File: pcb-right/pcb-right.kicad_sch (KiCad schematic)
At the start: 39 parts, among them J3 BAT, U2 xiao-ble

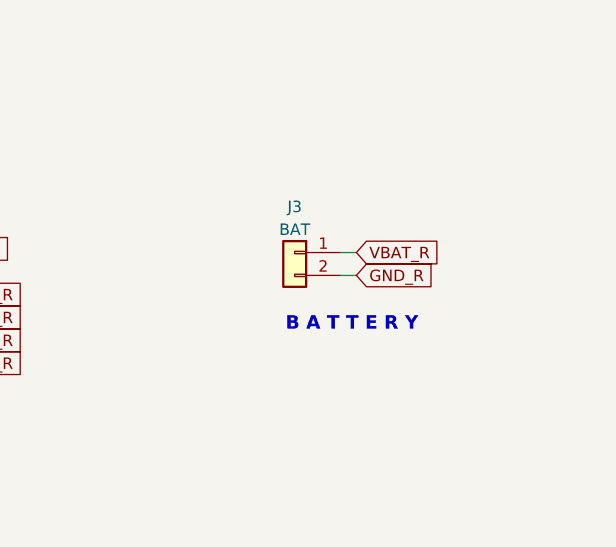
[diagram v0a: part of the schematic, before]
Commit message: Update schematic and pcb to rev 0.32
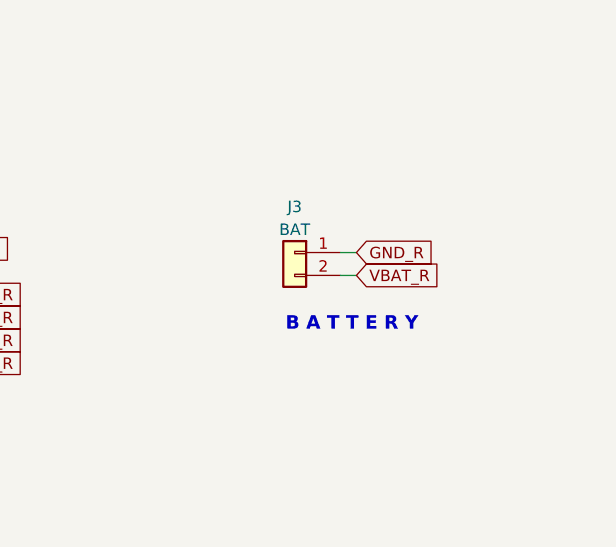
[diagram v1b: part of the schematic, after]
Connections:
- net GND_R: now also J3.1 (Pin_1); no longer J3.2 (Pin_2)
- net VBAT_R: now also J3.2 (Pin_2); no longer J3.1 (Pin_1)
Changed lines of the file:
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@@
     (title "Karma Wireless Split Ergonomic Keyboard")
     (date "2023-04-04")
-    (rev "0.1")
+    (rev "0.32")
   )
   (junction (at 150.1648 123.5964) (diameter 0) (color 0 0 0 0)
@@
     )
   )
-  (global_label "GND_R" (shape input) (at 152.4254 41.3512 0) (fields_autoplaced)
-    (effects (font (size 1.27 1.27)) (justify left))
-    (property "Intersheetrefs" "${INTERSHEET_REFS}" (at 161.4393 41.3512 0)
+  (global_label "VBAT_R" (shape input) (at 152.4254 41.3512 0) (fields_autoplaced)
+    (effects (font (size 1.27 1.27)) (justify left))
+    (property "Intersheetrefs" "${INTERSHEET_REFS}" (at 161.9836 41.3512 0)
       (effects (font (size 1.27 1.27)) (justify left) hide)
     )
@@
     )
   )
-  (global_label "VBAT_R" (shape input) (at 152.4254 38.8112 0) (fields_autoplaced)
-    (effects (font (size 1.27 1.27)) (justify left))
-    (property "Intersheetrefs" "${INTERSHEET_REFS}" (at 161.9836 38.8112 0)
+  (global_label "GND_R" (shape input) (at 152.4254 38.8112 0) (fields_autoplaced)
+    (effects (font (size 1.27 1.27)) (justify left))
+    (property "Intersheetrefs" "${INTERSHEET_REFS}" (at 161.4393 38.8112 0)
       (effects (font (size 1.27 1.27)) (justify left) hide)
     )
@@
         )
       )
-      (project "right-pcb"
+      (project "pcb-right"
         (path "/f98b87e5-a6a7-4c83-9bb9-aca334f9bfc8"
           (reference "DR8") (unit 1)
@@
         )
       )
-      (project "right-pcb"
+      (project "pcb-right"
         (path "/f98b87e5-a6a7-4c83-9bb9-aca334f9bfc8"
           (reference "DR2") (unit 1)
@@
         )
       )
-      (project "right-pcb"
+      (project "pcb-right"
         (path "/f98b87e5-a6a7-4c83-9bb9-aca334f9bfc8"
           (reference "DR6") (unit 1)
@@
         )
       )
-      (project "right-pcb"
+      (project "pcb-right"
         (path "/f98b87e5-a6a7-4c83-9bb9-aca334f9bfc8"
           (reference "SWR14") (unit 1)
@@
         )
       )
-      (project "right-pcb"
+      (project "pcb-right"
         (path "/f98b87e5-a6a7-4c83-9bb9-aca334f9bfc8"
           (reference "SWR8") (unit 1)
@@
         )
       )
-      (project "right-pcb"
+      (project "pcb-right"
         (path "/f98b87e5-a6a7-4c83-9bb9-aca334f9bfc8"
           (reference "SWR3") (unit 1)
@@
         )
       )
-      (project "right-pcb"
+      (project "pcb-right"
         (path "/f98b87e5-a6a7-4c83-9bb9-aca334f9bfc8"
           (reference "SWR12") (unit 1)
@@
         )
       )
-      (project "right-pcb"
+      (project "pcb-right"
         (path "/f98b87e5-a6a7-4c83-9bb9-aca334f9bfc8"
           (reference "DR12") (unit 1)
@@
         )
       )
-      (project "right-pcb"
+      (project "pcb-right"
         (path "/f98b87e5-a6a7-4c83-9bb9-aca334f9bfc8"
           (reference "DR13") (unit 1)
@@
         )
       )
-      (project "right-pcb"
+      (project "pcb-right"
         (path "/f98b87e5-a6a7-4c83-9bb9-aca334f9bfc8"
           (reference "SWR11") (unit 1)
@@
         )
       )
-      (project "right-pcb"
+      (project "pcb-right"
         (path "/f98b87e5-a6a7-4c83-9bb9-aca334f9bfc8"
           (reference "DR18") (unit 1)
@@
         )
       )
-      (project "right-pcb"
+      (project "pcb-right"
         (path "/f98b87e5-a6a7-4c83-9bb9-aca334f9bfc8"
           (reference "SWR16") (unit 1)
@@
         )
       )
-      (project "right-pcb"
+      (project "pcb-right"
         (path "/f98b87e5-a6a7-4c83-9bb9-aca334f9bfc8"
           (reference "DR11") (unit 1)
@@
         )
       )
-      (project "right-pcb"
+      (project "pcb-right"
         (path "/f98b87e5-a6a7-4c83-9bb9-aca334f9bfc8"
           (reference "DR4") (unit 1)
@@
         )
       )
-      (project "right-pcb"
+      (project "pcb-right"
         (path "/f98b87e5-a6a7-4c83-9bb9-aca334f9bfc8"
           (reference "SWR2") (unit 1)
@@
         )
       )
-      (project "right-pcb"
+      (project "pcb-right"
         (path "/f98b87e5-a6a7-4c83-9bb9-aca334f9bfc8"
           (reference "DR15") (unit 1)
@@
         )
       )
-      (project "right-pcb"
+      (project "pcb-right"
         (path "/f98b87e5-a6a7-4c83-9bb9-aca334f9bfc8"
           (reference "DR5") (unit 1)
@@
         )
       )
-      (project "right-pcb"
+      (project "pcb-right"
         (path "/f98b87e5-a6a7-4c83-9bb9-aca334f9bfc8"
           (reference "DR3") (unit 1)
@@
         )
       )
-      (project "right-pcb"
+      (project "pcb-right"
         (path "/f98b87e5-a6a7-4c83-9bb9-aca334f9bfc8"
           (reference "DR1") (unit 1)
@@
         )
       )
-      (project "right-pcb"
+      (project "pcb-right"
         (path "/f98b87e5-a6a7-4c83-9bb9-aca334f9bfc8"
           (reference "RSW2") (unit 1)
@@
         )
       )
-      (project "right-pcb"
+      (project "pcb-right"
         (path "/f98b87e5-a6a7-4c83-9bb9-aca334f9bfc8"
           (reference "SWR13") (unit 1)
@@
         )
       )
-      (project "right-pcb"
+      (project "pcb-right"
         (path "/f98b87e5-a6a7-4c83-9bb9-aca334f9bfc8"
           (reference "SWR6") (unit 1)
@@
         )
       )
-      (project "right-pcb"
+      (project "pcb-right"
         (path "/f98b87e5-a6a7-4c83-9bb9-aca334f9bfc8"
           (reference "DR7") (unit 1)
@@
         )
       )
-      (project "right-pcb"
+      (project "pcb-right"
         (path "/f98b87e5-a6a7-4c83-9bb9-aca334f9bfc8"
           (reference "SWR7") (unit 1)
@@
         )
       )
-      (project "right-pcb"
+      (project "pcb-right"
         (path "/f98b87e5-a6a7-4c83-9bb9-aca334f9bfc8"
           (reference "DR17") (unit 1)
@@
         )
       )
-      (project "right-pcb"
+      (project "pcb-right"
         (path "/f98b87e5-a6a7-4c83-9bb9-aca334f9bfc8"
           (reference "SWR4") (unit 1)
@@
         )
       )
-      (project "right-pcb"
+      (project "pcb-right"
         (path "/f98b87e5-a6a7-4c83-9bb9-aca334f9bfc8"
           (reference "J2") (unit 1)
@@
         )
       )
-      (project "right-pcb"
+      (project "pcb-right"
         (path "/f98b87e5-a6a7-4c83-9bb9-aca334f9bfc8"
           (reference "DR10") (unit 1)
@@
         )
       )
-      (project "right-pcb"
+      (project "pcb-right"
         (path "/f98b87e5-a6a7-4c83-9bb9-aca334f9bfc8"
           (reference "SWR10") (unit 1)
@@
         )
       )
-      (project "right-pcb"
+      (project "pcb-right"
         (path "/f98b87e5-a6a7-4c83-9bb9-aca334f9bfc8"
           (reference "DR14") (unit 1)
@@
         )
       )
-      (project "right-pcb"
+      (project "pcb-right"
         (path "/f98b87e5-a6a7-4c83-9bb9-aca334f9bfc8"
           (reference "DR9") (unit 1)
@@
         )
       )
-      (project "right-pcb"
+      (project "pcb-right"
         (path "/f98b87e5-a6a7-4c83-9bb9-aca334f9bfc8"
           (reference "SWR18") (unit 1)
@@
         )
       )
-      (project "right-pcb"
+      (project "pcb-right"
         (path "/f98b87e5-a6a7-4c83-9bb9-aca334f9bfc8"
           (reference "SWR9") (unit 1)
@@
         )
       )
-      (project "right-pcb"
+      (project "pcb-right"
         (path "/f98b87e5-a6a7-4c83-9bb9-aca334f9bfc8"
           (reference "SWR5") (unit 1)
@@
         )
       )
-      (project "right-pcb"
+      (project "pcb-right"
         (path "/f98b87e5-a6a7-4c83-9bb9-aca334f9bfc8"
           (reference "SWR17") (unit 1)
@@
         )
       )
-      (project "right-pcb"
+      (project "pcb-right"
         (path "/f98b87e5-a6a7-4c83-9bb9-aca334f9bfc8"
           (reference "U2") (unit 1)
@@
         )
       )
-      (project "right-pcb"
+      (project "pcb-right"
         (path "/f98b87e5-a6a7-4c83-9bb9-aca334f9bfc8"
           (reference "SWR1") (unit 1)
@@
         )
       )
-      (project "right-pcb"
+      (project "pcb-right"
         (path "/f98b87e5-a6a7-4c83-9bb9-aca334f9bfc8"
           (reference "SWR15") (unit 1)
@@
         )
       )
-      (project "right-pcb"
+      (project "pcb-right"
         (path "/f98b87e5-a6a7-4c83-9bb9-aca334f9bfc8"
           (reference "DR16") (unit 1)
